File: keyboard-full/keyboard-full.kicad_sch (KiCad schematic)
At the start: 372 parts, among them SW1 SW_Push, SW10 SW_Push, SW11 SW_Push, SW12 SW_Push, SW13 SW_Push, SW14 SW_Push, SW15 SW_Push, SW16 SW_Push, SW17 SW_Push, SW18 SW_Push, SW19 SW_Push, SW2 SW_Push, SW20 SW_Push, SW21 SW_Push, SW22 SW_Push, SW23 SW_Push, SW24 SW_Push, SW25 SW_Push, SW26 SW_Push, SW27 SW_Push, SW28 SW_Push, SW29 SW_Push, SW3 SW_Push, SW30 SW_Push, SW31 SW_Push, SW32 SW_Push, SW33 SW_Push, SW34 SW_Push, SW35 SW_Push, SW36 SW_Push, SW37 SW_Push, SW38 SW_Push, SW39 SW_Push, SW4 SW_Push, SW40 SW_Push, SW41 SW_Push, SW42 SW_Push, SW43 SW_Push, SW44 SW_Push, SW45 SW_Push, SW46 SW_Push, SW47 SW_Push, SW48 SW_Push, SW49 SW_Push, SW5 SW_Push, SW50 SW_Push, SW51 SW_Push, SW52 SW_Push, SW53 SW_Push, SW54 SW_Push, SW55 SW_Push, SW56 SW_Push, SW57 SW_Push, SW58 SW_Push, SW59 SW_Push, SW6 SW_Push, SW60 SW_Push, SW61 SW_Push, SW62 SW_Push, SW63 SW_Push, SW64 SW_Push, SW65 SW_Push, SW66 SW_Push, SW67 SW_Push, SW68 SW_Push, SW69 SW_Push, SW7 SW_Push, SW70 SW_Push, SW71 SW_Push, SW72 SW_Push, SW73 SW_Push, SW74 SW_Push, SW75 SW_Push, SW76 SW_Push, SW77 SW_Push, SW78 SW_Push, SW79 SW_Push, SW8 SW_Push, SW80 SW_Push, SW81 SW_Push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

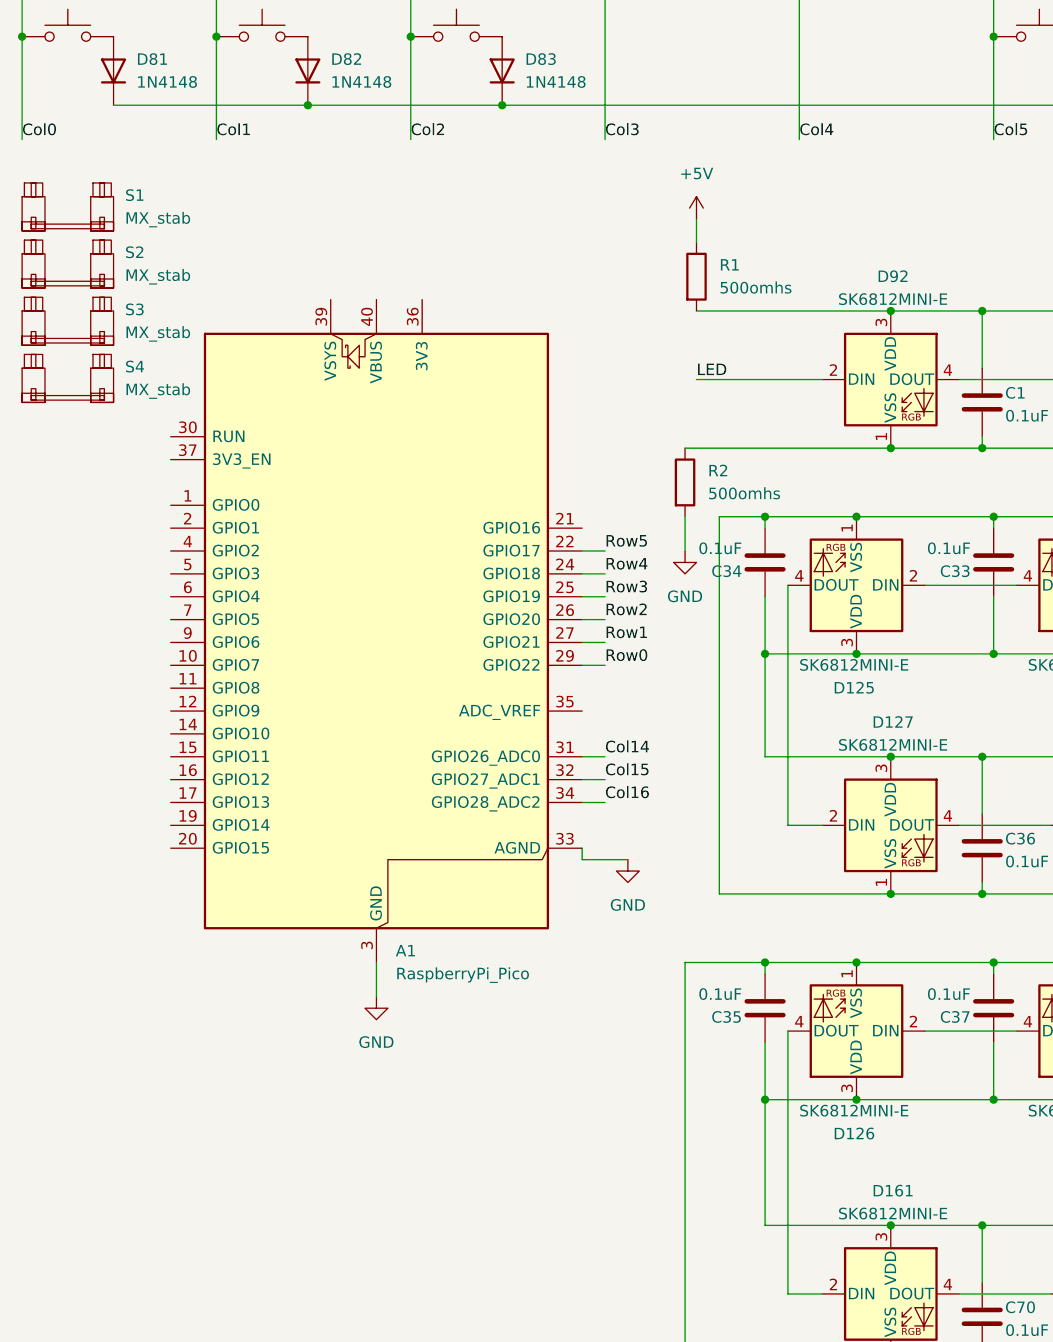
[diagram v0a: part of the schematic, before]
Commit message: Fixes to schema
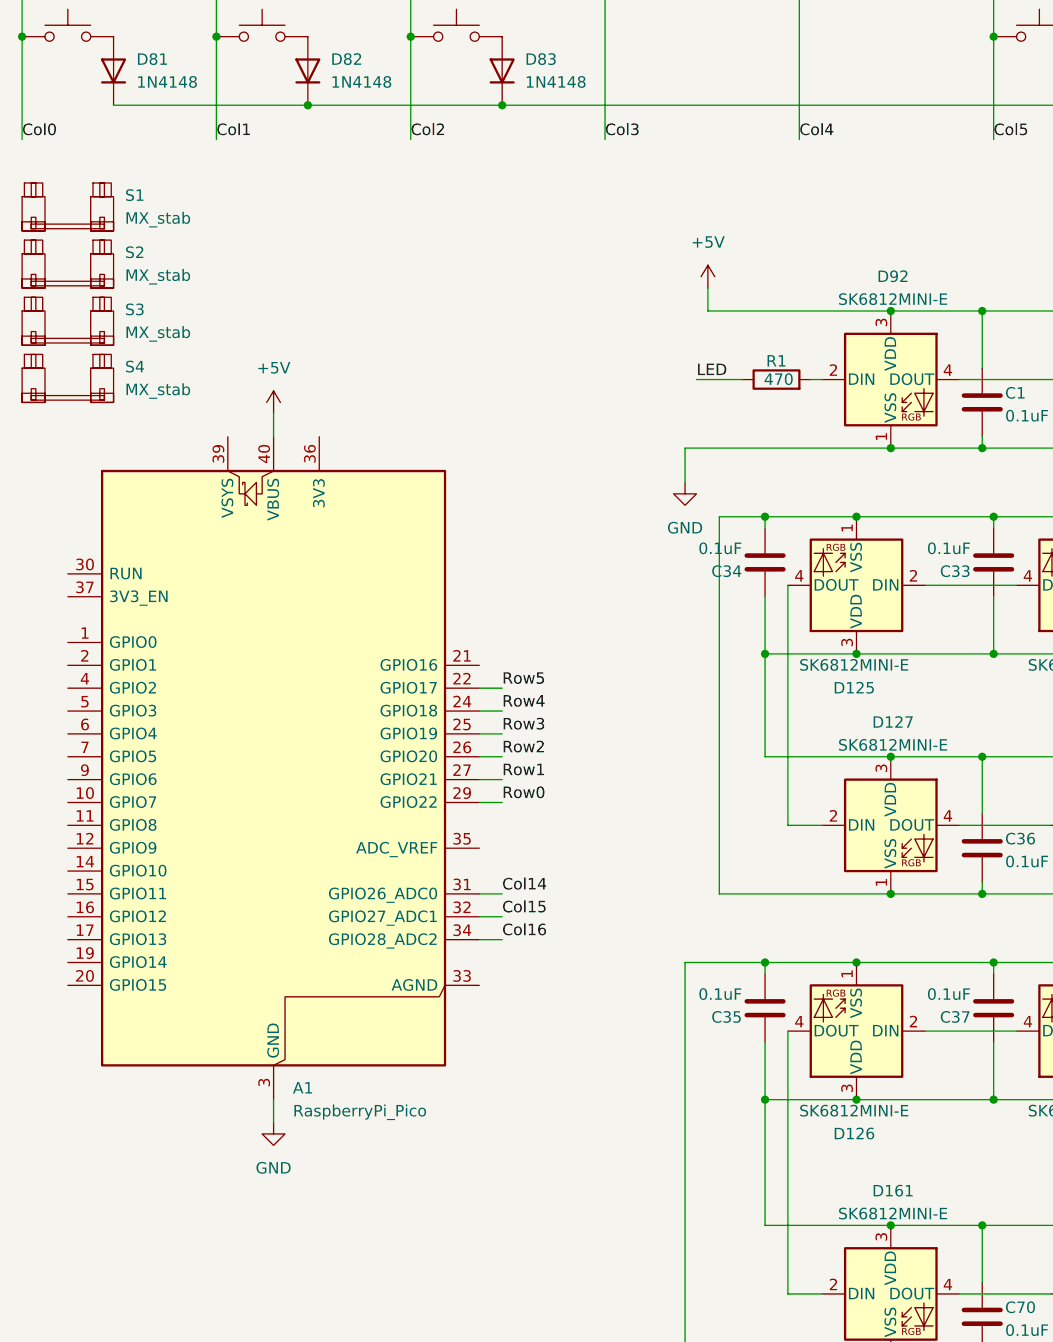
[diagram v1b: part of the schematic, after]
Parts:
- removed R2: 500omhs, symbol Device:R
- R1: value 500omhs -> 470
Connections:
- net +5V: now also A1.40 (VBUS), C1.1, C10.1, C100.1, C101.1, C102.1, C11.1, C12.1, C13.1, C14.1, C15.1, C16.1, C17.1, C18.1, C19.1, C20.1, C21.1, C22.1, C23.1, C24.1, C25.1, C26.1, C27.1, C28.1, C29.1, C3.1, C30.1, C31.1, C32.1, C33.1, C34.1, C35.1, C36.1, C37.1, C38.1, C39.1, C4.1, C40.1, C41.1, C42.1, C43.1, C44.1, C45.1, C46.1, C47.1, C48.1, C49.1, C5.1, C50.1, C51.1, C52.1, C53.1, C54.1, C55.1, C56.1, C57.1, C58.1, C59.1, C6.1, C60.1, C62.1, C63.1, C64.1, C66.1, C68.1, C69.1, C7.1, C70.1, C71.1, C72.1, C73.1, C74.1, C75.1, C76.1, C78.1, C8.1, C80.1, C81.1, C82.1, C84.1, C86.1, C88.1, C89.1, C9.1, C90.1, C91.1, C92.1, C93.1, C94.1, C96.1, C97.1, C98.1, C99.1, D100.3 (VDD), D101.3 (VDD), D102.3 (VDD), D103.3 (VDD), D104.3 (VDD), D105.3 (VDD), D106.3 (VDD), D107.3 (VDD), D108.3 (VDD), D109.3 (VDD), D110.3 (VDD), D111.3 (VDD), D112.3 (VDD), D113.3 (VDD), D114.3 (VDD), D115.3 (VDD), D116.3 (VDD), D117.3 (VDD), D118.3 (VDD), D119.3 (VDD), D120.3 (VDD), D121.3 (VDD), D122.3 (VDD), D123.3 (VDD), D124.3 (VDD), D125.3 (VDD), D126.3 (VDD), D127.3 (VDD), D128.3 (VDD), D129.3 (VDD), D130.3 (VDD), D131.3 (VDD), D132.3 (VDD), D133.3 (VDD), D134.3 (VDD), D135.3 (VDD), D136.3 (VDD), D137.3 (VDD), D138.3 (VDD), D139.3 (VDD), D140.3 (VDD), D141.3 (VDD), D142.3 (VDD), D143.3 (VDD), D144.3 (VDD), D145.3 (VDD), D146.3 (VDD), D147.3 (VDD), D148.3 (VDD), D149.3 (VDD), D151.3 (VDD), D152.3 (VDD), D153.3 (VDD), D155.3 (VDD), D157.3 (VDD), D159.3 (VDD), D160.3 (VDD), D161.3 (VDD), D162.3 (VDD), D163.3 (VDD), D164.3 (VDD), D165.3 (VDD), D167.3 (VDD), D169.3 (VDD), D170.3 (VDD), D171.3 (VDD), D173.3 (VDD), D175.3 (VDD), D177.3 (VDD), D178.3 (VDD), D179.3 (VDD), D180.3 (VDD), D181.3 (VDD), D182.3 (VDD), D183.3 (VDD), D185.3 (VDD), D186.3 (VDD), D187.3 (VDD), D188.3 (VDD), D189.3 (VDD), D190.3 (VDD), D191.3 (VDD), D192.3 (VDD), D193.3 (VDD), D92.3 (VDD), D94.3 (VDD), D95.3 (VDD), D96.3 (VDD), D97.3 (VDD), D98.3 (VDD), D99.3 (VDD); no longer R1.1
- net GND: now also C1.2, C10.2, C100.2, C101.2, C102.2, C11.2, C12.2, C13.2, C14.2, C15.2, C16.2, C17.2, C18.2, C19.2, C20.2, C21.2, C22.2, C23.2, C24.2, C25.2, C26.2, C27.2, C28.2, C29.2, C3.2, C30.2, C31.2, C32.2, C33.2, C34.2, C35.2, C36.2, C37.2, C38.2, C39.2, C4.2, C40.2, C41.2, C42.2, C43.2, C44.2, C45.2, C46.2, C47.2, C48.2, C49.2, C5.2, C50.2, C51.2, C52.2, C53.2, C54.2, C55.2, C56.2, C57.2, C58.2, C59.2, C6.2, C60.2, C62.2, C63.2, C64.2, C66.2, C68.2, C69.2, C7.2, C70.2, C71.2, C72.2, C73.2, C74.2, C75.2, C76.2, C78.2, C8.2, C80.2, C81.2, C82.2, C84.2, C86.2, C88.2, C89.2, C9.2, C90.2, C91.2, C92.2, C93.2, C94.2, C96.2, C97.2, C98.2, C99.2, D100.1 (VSS), D101.1 (VSS), D102.1 (VSS), D103.1 (VSS), D104.1 (VSS), D105.1 (VSS), D106.1 (VSS), D107.1 (VSS), D108.1 (VSS), D109.1 (VSS), D110.1 (VSS), D111.1 (VSS), D112.1 (VSS), D113.1 (VSS), D114.1 (VSS), D115.1 (VSS), D116.1 (VSS), D117.1 (VSS), D118.1 (VSS), D119.1 (VSS), D120.1 (VSS), D121.1 (VSS), D122.1 (VSS), D123.1 (VSS), D124.1 (VSS), D125.1 (VSS), D126.1 (VSS), D127.1 (VSS), D128.1 (VSS), D129.1 (VSS), D130.1 (VSS), D131.1 (VSS), D132.1 (VSS), D133.1 (VSS), D134.1 (VSS), D135.1 (VSS), D136.1 (VSS), D137.1 (VSS), D138.1 (VSS), D139.1 (VSS), D140.1 (VSS), D141.1 (VSS), D142.1 (VSS), D143.1 (VSS), D144.1 (VSS), D145.1 (VSS), D146.1 (VSS), D147.1 (VSS), D148.1 (VSS), D149.1 (VSS), D151.1 (VSS), D152.1 (VSS), D153.1 (VSS), D155.1 (VSS), D157.1 (VSS), D159.1 (VSS), D160.1 (VSS), D161.1 (VSS), D162.1 (VSS), D163.1 (VSS), D164.1 (VSS), D165.1 (VSS), D167.1 (VSS), D169.1 (VSS), D170.1 (VSS), D171.1 (VSS), D173.1 (VSS), D175.1 (VSS), D177.1 (VSS), D178.1 (VSS), D179.1 (VSS), D180.1 (VSS), D181.1 (VSS), D182.1 (VSS), D183.1 (VSS), D185.1 (VSS), D186.1 (VSS), D187.1 (VSS), D188.1 (VSS), D189.1 (VSS), D190.1 (VSS), D191.1 (VSS), D192.1 (VSS), D193.1 (VSS), D92.1 (VSS), D94.1 (VSS), D95.1 (VSS), D96.1 (VSS), D97.1 (VSS), D98.1 (VSS), D99.1 (VSS); no longer A1.33 (AGND)
- net LED: now also R1.1; no longer D92.2 (DIN)
- new net: D92.2 (DIN), R1.2
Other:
- moved on the sheet: A1

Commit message: progress on keyboard
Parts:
- removed C100, C101, C102, C92, C93, C94, C96, C97, C98, C99: 0.1uF, symbol Device:C
- removed D109, D110, D111, D112, D113, D114, D115, D116, D117, D118, D119, D120, D121, D122, D123, D124, D125, D126, D127, D128, D129, D130, D131, D132, D133, D134, D135, D136, D137, D138, D139, D140, D141, D142, D143, D144, D145, D146, D147, D148, D149, D151, D152, D153, D155, D157, D159, D160, D161, D162, D163, D164, D165, D167, D169, D170, D171, D173, D175, D177, D178, D179, D180, D181, D182, D183, D185, D186, D187, D188, D189, D190, D191, D192, D193: SK6812MINI-E, LED_SMD:LED_SK6812MINI-E_3.2x2.8mm_P1.5mm_ReverseMount, symbol LED:SK6812MINI-E
- removed SW1, SW10, SW11, SW12, SW13, SW14, SW15, SW16, SW17, SW18, SW19, SW2, SW20, SW21, SW22, SW23, SW24, SW25, SW26, SW27, SW28, SW29, SW3, SW30, SW31, SW32, SW33, SW34, SW35, SW36, SW37, SW38, SW39, SW4, SW40, SW41, SW42, SW43, SW44, SW45, SW46, SW47, SW48, SW49, SW5, SW50, SW51, SW52, SW53, SW54, SW55, SW56, SW57, SW58, SW59, SW6, SW60, SW61, SW62, SW63, SW64, SW65, SW66, SW67, SW68, SW69, SW7, SW70, SW71, SW72, SW73, SW74, SW75, SW76, SW77, SW78, SW79, SW8, SW80, SW81, SW82, SW83, SW85, SW86, SW87, SW88, SW89, SW9, SW90, SW91: SW_Push, PCM_marbastlib-mx:SW_MX_1u, symbol Switch:SW_Push
- removed SW84: SW_Push, PCM_marbastlib-mx:STAB_MX_P_6u, symbol Switch:SW_Push
- added C17, C61, C65, C67, C77, C79, C83, C85, C87: 0.1uF, Capacitor_SMD:C_1206_3216Metric_Pad1.33x1.80mm_HandSolder, symbol Device:C
- added H1, H2, H3, H4: MountingHole, MountingHole:MountingHole_2.1mm, symbol Mechanical:MountingHole
- added LED17, LED18, LED19, LED20, LED21, LED22, LED23, LED24, LED25, LED26, LED27, LED28, LED29, LED30, LED31, LED32, LED33, LED34, LED35, LED36, LED37, LED38, LED39, LED40, LED41, LED42, LED43, LED44, LED45, LED46, LED47, LED48, LED49, LED50, LED51, LED52, LED53, LED54, LED55, LED56, LED57, LED58, LED59, LED60, LED61, LED62, LED63, LED64, LED65, LED66, LED67, LED68, LED69, LED70, LED71, LED72, LED73, LED74, LED75, LED76, LED77, LED78, LED79, LED80, LED81, LED82, LED83, LED84, LED85, LED86, LED87, LED88, LED89, LED90, LED91: SK6812MINI-E, LED_SMD:LED_SK6812MINI-E_3.2x2.8mm_P1.5mm_ReverseMount, symbol LED:SK6812MINI-E
- added MX1, MX10, MX11, MX12, MX13, MX14, MX15, MX16, MX17, MX18, MX19, MX2, MX20, MX21, MX22, MX23, MX24, MX25, MX26, MX27, MX28, MX29, MX3, MX30, MX31, MX32, MX33, MX35, MX36, MX37, MX38, MX39, MX4, MX40, MX41, MX42, MX43, MX44, MX45, MX46, MX48, MX49, MX5, MX50, MX52, MX53, MX54, MX55, MX56, MX57, MX58, MX59, MX6, MX60, MX61, MX62, MX63, MX64, MX65, MX66, MX67, MX68, MX69, MX7, MX70, MX71, MX72, MX73, MX74, MX75, MX76, MX77, MX78, MX79, MX8, MX80, MX89, MX9, MX90, MX91: MX_SW_HS, PCM_marbastlib-mx:SW_MX_HS_CPG151101S11_1u, symbol PCM_marbastlib-mx:MX_SW_HS_CPG151101S11
- added MX34: MX_SW_HS, PCM_marbastlib-mx:SW_MX_HS_CPG151101S11_1.5u, symbol PCM_marbastlib-mx:MX_SW_HS_CPG151101S11
- added MX47: MX_SW_HS, PCM_marbastlib-mx:SW_MX_HS_KS-2P02B01-01_1.5u, symbol PCM_marbastlib-mx:MX_SW_HS_CPG151101S11
- added MX51: MX_SW_HS, PCM_marbastlib-mx:SW_MX_HS_KS-2P02B01-01_1.75u, symbol PCM_marbastlib-mx:MX_SW_HS_CPG151101S11
- added MX81, MX82, MX83, MX85, MX86, MX87, MX88: MX_SW_HS, PCM_marbastlib-mx:SW_MX_HS_KS-2P02B01-01_1.25u, symbol PCM_marbastlib-mx:MX_SW_HS_CPG151101S11
- added MX84: MX_SW_HS, PCM_marbastlib-mx:SW_MX_HS_CPG151101S11_1.25u, symbol PCM_marbastlib-mx:MX_SW_HS_CPG151101S11
- C1, C18, C19, C20, C21, C22, C23, C24, C25, C26, C27, C28, C29, C30, C31, C32, C33, C34, C35, C36, C37, C38, C39, C40, C41, C42, C43, C44, C45, C46, C47, C48, C49, C50, C51, C52, C53, C54, C55, C56, C57, C58, C59, C60, C62, C63, C64, C66, C68, C69, C70, C71, C72, C73, C74, C75, C76, C78, C80, C81, C82, C84, C86, C88, C89, C90, C91: footprint (none) -> Capacitor_SMD:C_1206_3216Metric_Pad1.33x1.80mm_HandSolder
- C10: renamed from C11; footprint (none) -> Capacitor_SMD:C_1206_3216Metric_Pad1.33x1.80mm_HandSolder
- C11: renamed from C12; footprint (none) -> Capacitor_SMD:C_1206_3216Metric_Pad1.33x1.80mm_HandSolder
- C12: renamed from C13; footprint (none) -> Capacitor_SMD:C_1206_3216Metric_Pad1.33x1.80mm_HandSolder
- C13: renamed from C14; footprint (none) -> Capacitor_SMD:C_1206_3216Metric_Pad1.33x1.80mm_HandSolder
- C14: renamed from C15; footprint (none) -> Capacitor_SMD:C_1206_3216Metric_Pad1.33x1.80mm_HandSolder
- C15: renamed from C16; footprint (none) -> Capacitor_SMD:C_1206_3216Metric_Pad1.33x1.80mm_HandSolder
- C16: renamed from C17; footprint (none) -> Capacitor_SMD:C_1206_3216Metric_Pad1.33x1.80mm_HandSolder
- C2: renamed from C3; footprint (none) -> Capacitor_SMD:C_1206_3216Metric_Pad1.33x1.80mm_HandSolder
- C3: renamed from C4; footprint (none) -> Capacitor_SMD:C_1206_3216Metric_Pad1.33x1.80mm_HandSolder
- C4: renamed from C5; footprint (none) -> Capacitor_SMD:C_1206_3216Metric_Pad1.33x1.80mm_HandSolder
- C5: renamed from C6; footprint (none) -> Capacitor_SMD:C_1206_3216Metric_Pad1.33x1.80mm_HandSolder
- C6: renamed from C7; footprint (none) -> Capacitor_SMD:C_1206_3216Metric_Pad1.33x1.80mm_HandSolder
- C7: renamed from C8; footprint (none) -> Capacitor_SMD:C_1206_3216Metric_Pad1.33x1.80mm_HandSolder
- C8: renamed from C9; footprint (none) -> Capacitor_SMD:C_1206_3216Metric_Pad1.33x1.80mm_HandSolder
- C9: renamed from C10; footprint (none) -> Capacitor_SMD:C_1206_3216Metric_Pad1.33x1.80mm_HandSolder
- R1: footprint (none) -> Resistor_THT:R_Axial_DIN0207_L6.3mm_D2.5mm_P7.62mm_Horizontal
- S2, S3: footprint PCM_marbastlib-mx:STAB_MX_P_6.25u -> PCM_marbastlib-mx:STAB_MX_2u
- S4: footprint PCM_marbastlib-mx:STAB_MX_P_6.25u -> PCM_marbastlib-mx:STAB_MX_2.25u
- renumbered D92 to LED1, D102 to LED10, D103 to LED11, D104 to LED12, D105 to LED13, D106 to LED14, D107 to LED15, D108 to LED16, D94 to LED2, D95 to LED3, D96 to LED4, D97 to LED5, D98 to LED6, D99 to LED7, D100 to LED8, D101 to LED9
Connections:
- net +5V: now also C17.1, C61.1, C65.1, C67.1, C77.1, C79.1, C83.1, C85.1, C87.1, LED17.3 (VDD), LED18.3 (VDD), LED19.3 (VDD), LED20.3 (VDD), LED21.3 (VDD), LED22.3 (VDD), LED23.3 (VDD), LED24.3 (VDD), LED25.3 (VDD), LED26.3 (VDD), LED27.3 (VDD), LED28.3 (VDD), LED29.3 (VDD), LED30.3 (VDD), LED31.3 (VDD), LED32.3 (VDD), LED33.3 (VDD), LED34.3 (VDD), LED35.3 (VDD), LED36.3 (VDD), LED37.3 (VDD), LED38.3 (VDD), LED39.3 (VDD), LED40.3 (VDD), LED41.3 (VDD), LED42.3 (VDD), LED43.3 (VDD), LED44.3 (VDD), LED45.3 (VDD), LED46.3 (VDD), LED47.3 (VDD), LED48.3 (VDD), LED49.3 (VDD), LED50.3 (VDD), LED51.3 (VDD), LED52.3 (VDD), LED53.3 (VDD), LED54.3 (VDD), LED55.3 (VDD), LED56.3 (VDD), LED57.3 (VDD), LED58.3 (VDD), LED59.3 (VDD), LED60.3 (VDD), LED61.3 (VDD), LED62.3 (VDD), LED63.3 (VDD), LED64.3 (VDD), LED65.3 (VDD), LED66.3 (VDD), LED67.3 (VDD), LED68.3 (VDD), LED69.3 (VDD), LED70.3 (VDD), LED71.3 (VDD), LED72.3 (VDD), LED73.3 (VDD), LED74.3 (VDD), LED75.3 (VDD), LED76.3 (VDD), LED77.3 (VDD), LED78.3 (VDD), LED79.3 (VDD), LED80.3 (VDD), LED81.3 (VDD), LED82.3 (VDD), LED83.3 (VDD), LED84.3 (VDD), LED85.3 (VDD), LED86.3 (VDD), LED87.3 (VDD), LED88.3 (VDD), LED89.3 (VDD), LED90.3 (VDD), LED91.3 (VDD)
- net Col0: now also MX1.1, MX17.1, MX34.1, MX51.1, MX64.1, MX81.1
- net Col1: now also MX18.1, MX35.1, MX52.1, MX65.1, MX82.1
- net Col10: now also MX10.1, MX27.1, MX44.1, MX61.1, MX74.1, MX86.1
- net Col11: now also MX11.1, MX28.1, MX45.1, MX62.1, MX75.1, MX87.1
- net Col12: now also MX12.1, MX29.1, MX46.1, MX76.1
- net Col13: now also MX13.1, MX30.1, MX47.1, MX63.1, MX77.1, MX88.1
- net Col14: now also MX14.1, MX31.1, MX48.1, MX78.1, MX89.1
- net Col15: now also MX15.1, MX32.1, MX49.1, MX79.1, MX90.1
- net Col16: now also MX16.1, MX33.1, MX50.1, MX80.1, MX91.1
- net Col2: now also MX19.1, MX2.1, MX36.1, MX53.1, MX66.1, MX83.1
- net Col3: now also MX20.1, MX3.1, MX37.1, MX54.1, MX67.1
- net Col4: now also MX21.1, MX38.1, MX4.1, MX55.1, MX68.1
- net Col5: now also MX22.1, MX39.1, MX5.1, MX56.1, MX69.1, MX84.1
- net Col6: now also MX23.1, MX40.1, MX57.1, MX6.1, MX70.1
- net Col7: now also MX24.1, MX41.1, MX58.1, MX7.1, MX71.1
- net Col8: now also MX25.1, MX42.1, MX59.1, MX72.1, MX8.1
- net Col9: now also MX26.1, MX43.1, MX60.1, MX73.1, MX85.1, MX9.1
- net GND: now also C17.2, C61.2, C65.2, C67.2, C77.2, C79.2, C83.2, C85.2, C87.2, LED17.1 (VSS), LED18.1 (VSS), LED19.1 (VSS), LED20.1 (VSS), LED21.1 (VSS), LED22.1 (VSS), LED23.1 (VSS), LED24.1 (VSS), LED25.1 (VSS), LED26.1 (VSS), LED27.1 (VSS), LED28.1 (VSS), LED29.1 (VSS), LED30.1 (VSS), LED31.1 (VSS), LED32.1 (VSS), LED33.1 (VSS), LED34.1 (VSS), LED35.1 (VSS), LED36.1 (VSS), LED37.1 (VSS), LED38.1 (VSS), LED39.1 (VSS), LED40.1 (VSS), LED41.1 (VSS), LED42.1 (VSS), LED43.1 (VSS), LED44.1 (VSS), LED45.1 (VSS), LED46.1 (VSS), LED47.1 (VSS), LED48.1 (VSS), LED49.1 (VSS), LED50.1 (VSS), LED51.1 (VSS), LED52.1 (VSS), LED53.1 (VSS), LED54.1 (VSS), LED55.1 (VSS), LED56.1 (VSS), LED57.1 (VSS), LED58.1 (VSS), LED59.1 (VSS), LED60.1 (VSS), LED61.1 (VSS), LED62.1 (VSS), LED63.1 (VSS), LED64.1 (VSS), LED65.1 (VSS), LED66.1 (VSS), LED67.1 (VSS), LED68.1 (VSS), LED69.1 (VSS), LED70.1 (VSS), LED71.1 (VSS), LED72.1 (VSS), LED73.1 (VSS), LED74.1 (VSS), LED75.1 (VSS), LED76.1 (VSS), LED77.1 (VSS), LED78.1 (VSS), LED79.1 (VSS), LED80.1 (VSS), LED81.1 (VSS), LED82.1 (VSS), LED83.1 (VSS), LED84.1 (VSS), LED85.1 (VSS), LED86.1 (VSS), LED87.1 (VSS), LED88.1 (VSS), LED89.1 (VSS), LED90.1 (VSS), LED91.1 (VSS)
- net at D30.2 (A): now also MX30.2
- net at D86.2 (A): now also MX86.2
- net at D36.2 (A): now also MX36.2
- net at D68.2 (A): now also MX68.2
- net at D78.2 (A): now also MX78.2
- net at D21.2 (A): now also MX21.2
- net at D72.2 (A): now also MX72.2
- net at D35.2 (A): now also MX35.2
- net at D54.2 (A): now also MX54.2
- net at D81.2 (A): now also MX81.2
- net at D62.2 (A): now also MX62.2
- net at D70.2 (A): now also MX70.2
- net at D29.2 (A): now also MX29.2
- net at D57.2 (A): now also MX57.2
- net at D76.2 (A): now also MX76.2
- net at D56.2 (A): now also MX56.2
- net at D26.2 (A): now also MX26.2
- net at D88.2 (A): now also MX88.2
- net at D66.2 (A): now also MX66.2
- net at D6.2 (A): now also MX6.2
- net at D49.2 (A): now also MX49.2
- net at D1.2 (A): now also MX1.2
- net at D33.2 (A): now also MX33.2
- net at D37.2 (A): now also MX37.2
- net at D48.2 (A): now also MX48.2
- net at D75.2 (A): now also MX75.2
- net at D90.2 (A): now also MX90.2
- net at D79.2 (A): now also MX79.2
- net at D74.2 (A): now also MX74.2
- net at D22.2 (A): now also MX22.2
- net at D28.2 (A): now also MX28.2
- net at D15.2 (A): now also MX15.2
- net at D2.2 (A): now also MX2.2
- net at D85.2 (A): now also MX85.2
- net at D23.2 (A): now also MX23.2
- net at D7.2 (A): now also MX7.2
- net at D55.2 (A): now also MX55.2
- net at D9.2 (A): now also MX9.2
- net at D44.2 (A): now also MX44.2
- net at D41.2 (A): now also MX41.2
- net at D67.2 (A): now also MX67.2
- net at D65.2 (A): now also MX65.2
- net at D77.2 (A): now also MX77.2
- net at D17.2 (A): now also MX17.2
- net at D31.2 (A): now also MX31.2
- net at D8.2 (A): now also MX8.2
- net at D91.2 (A): now also MX91.2
- net at D34.2 (A): now also MX34.2
- net at D27.2 (A): now also MX27.2
- net at D4.2 (A): now also MX4.2
- net at D32.2 (A): now also MX32.2
- net at D24.2 (A): now also MX24.2
- net at D38.2 (A): now also MX38.2
- net at D5.2 (A): now also MX5.2
- net at D89.2 (A): now also MX89.2
- net at D50.2 (A): now also MX50.2
- net at D42.2 (A): now also MX42.2
- net at LED16.4 (DOUT): now also LED17.2 (DIN)
- net at D59.2 (A): now also MX59.2
- net at D10.2 (A): now also MX10.2
- net at D69.2 (A): now also MX69.2
- net at D73.2 (A): now also MX73.2
- net at D46.2 (A): now also MX46.2
- net at D13.2 (A): now also MX13.2
- net at D53.2 (A): now also MX53.2
- net at D12.2 (A): now also MX12.2
- net at D52.2 (A): now also MX52.2
- net at D84.2 (A): now also MX84.2
- net at D45.2 (A): now also MX45.2
- net at D58.2 (A): now also MX58.2
- net at D83.2 (A): now also MX83.2
- net at D3.2 (A): now also MX3.2
- net at D39.2 (A): now also MX39.2
- net at D47.2 (A): now also MX47.2
- net at D11.2 (A): now also MX11.2
- net at D71.2 (A): now also MX71.2
- net at D61.2 (A): now also MX61.2
- net at D63.2 (A): now also MX63.2
- net at D82.2 (A): now also MX82.2
- net at D51.2 (A): now also MX51.2
- net at D14.2 (A): now also MX14.2
- net at D25.2 (A): now also MX25.2
- net at D18.2 (A): now also MX18.2
- net at D19.2 (A): now also MX19.2
- net at D60.2 (A): now also MX60.2
- net at D40.2 (A): now also MX40.2
- net at D87.2 (A): now also MX87.2
- net at D16.2 (A): now also MX16.2
- net at D64.2 (A): now also MX64.2
- net at D80.2 (A): now also MX80.2
- net at D20.2 (A): now also MX20.2
- net at D43.2 (A): now also MX43.2
- new net: LED42.4 (DOUT), LED43.2 (DIN)
- new net: LED43.4 (DOUT), LED44.2 (DIN)
- new net: LED38.4 (DOUT), LED39.2 (DIN)
- new net: LED39.4 (DOUT), LED40.2 (DIN)
- new net: LED60.4 (DOUT), LED61.2 (DIN)
- new net: LED61.4 (DOUT), LED62.2 (DIN)
- new net: LED64.4 (DOUT), LED65.2 (DIN)
- new net: LED65.4 (DOUT), LED66.2 (DIN)
- new net: LED62.4 (DOUT), LED63.2 (DIN)
- new net: LED63.4 (DOUT), LED64.2 (DIN)
- new net: LED24.4 (DOUT), LED25.2 (DIN)
- new net: LED25.4 (DOUT), LED26.2 (DIN)
- new net: LED47.4 (DOUT), LED48.2 (DIN)
- new net: LED48.4 (DOUT), LED49.2 (DIN)
- new net: LED35.4 (DOUT), LED36.2 (DIN)
- new net: LED36.4 (DOUT), LED37.2 (DIN)
- new net: LED22.4 (DOUT), LED23.2 (DIN)
- new net: LED23.4 (DOUT), LED24.2 (DIN)
- new net: LED76.4 (DOUT), LED77.2 (DIN)
- new net: LED77.4 (DOUT), LED78.2 (DIN)
- new net: LED89.4 (DOUT), LED90.2 (DIN)
- new net: LED90.4 (DOUT), LED91.2 (DIN)
- new net: LED66.4 (DOUT), LED67.2 (DIN)
- new net: LED67.4 (DOUT), LED68.2 (DIN)
- new net: LED85.4 (DOUT), LED86.2 (DIN)
- new net: LED86.4 (DOUT), LED87.2 (DIN)
- new net: LED57.4 (DOUT), LED58.2 (DIN)
- new net: LED58.4 (DOUT), LED59.2 (DIN)
- new net: LED20.4 (DOUT), LED21.2 (DIN)
- new net: LED21.4 (DOUT), LED22.2 (DIN)
- new net: LED40.4 (DOUT), LED41.2 (DIN)
- new net: LED44.4 (DOUT), LED45.2 (DIN)
- new net: LED45.4 (DOUT), LED46.2 (DIN)
- new net: LED50.4 (DOUT), LED51.2 (DIN)
- new net: LED51.4 (DOUT), LED52.2 (DIN)
- new net: LED26.4 (DOUT), LED27.2 (DIN)
- new net: LED27.4 (DOUT), LED28.2 (DIN)
- new net: LED46.4 (DOUT), LED47.2 (DIN)
- new net: LED87.4 (DOUT), LED88.2 (DIN)
- new net: LED17.4 (DOUT), LED18.2 (DIN)
- new net: LED41.4 (DOUT), LED42.2 (DIN)
- new net: LED82.4 (DOUT), LED83.2 (DIN)
- new net: LED83.4 (DOUT), LED84.2 (DIN)
- new net: LED28.4 (DOUT), LED29.2 (DIN)
- new net: LED37.4 (DOUT), LED38.2 (DIN)
- new net: LED78.4 (DOUT), LED79.2 (DIN)
- new net: LED59.4 (DOUT), LED60.2 (DIN)
- new net: LED68.4 (DOUT), LED69.2 (DIN)
- new net: LED54.4 (DOUT), LED55.2 (DIN)
- new net: LED55.4 (DOUT), LED56.2 (DIN)
- new net: LED19.4 (DOUT), LED20.2 (DIN)
- new net: LED79.4 (DOUT), LED80.2 (DIN)
- new net: LED80.4 (DOUT), LED81.2 (DIN)
- new net: LED81.4 (DOUT), LED82.2 (DIN)
- new net: LED71.4 (DOUT), LED72.2 (DIN)
- new net: LED72.4 (DOUT), LED73.2 (DIN)
- new net: LED33.4 (DOUT), LED34.2 (DIN)
- new net: LED34.4 (DOUT), LED35.2 (DIN)
- new net: LED70.4 (DOUT), LED71.2 (DIN)
- new net: LED49.4 (DOUT), LED50.2 (DIN)
- new net: LED56.4 (DOUT), LED57.2 (DIN)
- new net: LED53.4 (DOUT), LED54.2 (DIN)
- new net: LED84.4 (DOUT), LED85.2 (DIN)
- new net: LED18.4 (DOUT), LED19.2 (DIN)
- new net: LED75.4 (DOUT), LED76.2 (DIN)
- new net: LED73.4 (DOUT), LED74.2 (DIN)
- new net: LED74.4 (DOUT), LED75.2 (DIN)
- new net: LED30.4 (DOUT), LED31.2 (DIN)
- new net: LED31.4 (DOUT), LED32.2 (DIN)
- new net: LED69.4 (DOUT), LED70.2 (DIN)
- new net: LED32.4 (DOUT), LED33.2 (DIN)
- new net: LED52.4 (DOUT), LED53.2 (DIN)
- new net: LED29.4 (DOUT), LED30.2 (DIN)
- new net: LED88.4 (DOUT), LED89.2 (DIN)
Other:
- moved on the sheet: A1, C1, C10, C11, C12, C13, C14, C15, C16, C2, C3, C4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

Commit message: Started wiring, and fixed pcb's rgbs data line going across the whole board
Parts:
- added C100, C101, C102, C92, C93, C94, C95, C96, C97, C98, C99: 0.1uF, Capacitor_SMD:C_1206_3216Metric_Pad1.33x1.80mm_HandSolder, symbol Device:C
- added LED100, LED101, LED102, LED92, LED93, LED94, LED95, LED96, LED97, LED98, LED99: SK6812MINI-E, LED_SMD:LED_SK6812MINI-E_3.2x2.8mm_P1.5mm_ReverseMount, symbol LED:SK6812MINI-E
- S1: footprint PCM_marbastlib-mx:STAB_MX_P_6.25u -> PCM_marbastlib-mx:STAB_MX_6.25u
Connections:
- net +5V: now also C100.1, C101.1, C102.1, C92.1, C93.1, C94.1, C95.1, C96.1, C97.1, C98.1, C99.1, LED100.3 (VDD), LED101.3 (VDD), LED102.3 (VDD), LED92.3 (VDD), LED93.3 (VDD), LED94.3 (VDD), LED95.3 (VDD), LED96.3 (VDD), LED97.3 (VDD), LED98.3 (VDD), LED99.3 (VDD)
- net GND: now also C100.2, C101.2, C102.2, C92.2, C93.2, C94.2, C95.2, C96.2, C97.2, C98.2, C99.2, LED100.1 (VSS), LED101.1 (VSS), LED102.1 (VSS), LED92.1 (VSS), LED93.1 (VSS), LED94.1 (VSS), LED95.1 (VSS), LED96.1 (VSS), LED97.1 (VSS), LED98.1 (VSS), LED99.1 (VSS)
- net at LED43.2 (DIN): now also LED41.4 (DOUT); no longer LED42.4 (DOUT)
- net at LED43.4 (DOUT): now also LED45.2 (DIN); no longer LED44.2 (DIN)
- net at LED38.4 (DOUT): now also LED36.2 (DIN); no longer LED39.2 (DIN)
- net at LED39.4 (DOUT): now also LED41.2 (DIN); no longer LED40.2 (DIN)
- net at LED60.4 (DOUT): now also LED58.2 (DIN); no longer LED61.2 (DIN)
- net at LED62.2 (DIN): now also LED64.4 (DOUT); no longer LED61.4 (DOUT)
- net at LED1.4 (DOUT): now also LED17.2 (DIN); no longer LED2.2 (DIN)
- net at LED65.2 (DIN): now also LED63.4 (DOUT); no longer LED64.4 (DOUT)
- net at LED66.2 (DIN): now also LED68.4 (DOUT); no longer LED65.4 (DOUT)
- net at LED62.4 (DOUT): now also LED60.2 (DIN); no longer LED63.2 (DIN)
- net at LED64.2 (DIN): now also LED66.4 (DOUT); no longer LED63.4 (DOUT)
- net at LED48.2 (DIN): now also LED50.4 (DOUT); no longer LED47.4 (DOUT)
- net at LED48.4 (DOUT): now also LED46.2 (DIN); no longer LED49.2 (DIN)
- net at LED35.4 (DOUT): now also LED37.2 (DIN); no longer LED36.2 (DIN)
- net at LED36.4 (DOUT): now also LED69.2 (DIN); no longer LED37.2 (DIN)
- net at LED76.4 (DOUT): now also LED74.2 (DIN); no longer LED77.2 (DIN)
- net at LED77.4 (DOUT): now also LED79.2 (DIN); no longer LED78.2 (DIN)
- net at LED89.4 (DOUT): now also LED91.2 (DIN); no longer LED90.2 (DIN)
- net at LED90.4 (DOUT): now also LED88.2 (DIN); no longer LED91.2 (DIN)
- net at LED67.2 (DIN): now also LED65.4 (DOUT); no longer LED66.4 (DOUT)
- net at LED86.2 (DIN): now also LED88.4 (DOUT); no longer LED85.4 (DOUT)
- net at LED86.4 (DOUT): now also LED84.2 (DIN); no longer LED87.2 (DIN)
- net at LED57.4 (DOUT): now also LED59.2 (DIN); no longer LED58.2 (DIN)
- net at LED58.4 (DOUT): now also LED56.2 (DIN); no longer LED59.2 (DIN)
- net at LED40.4 (DOUT): now also LED38.2 (DIN); no longer LED41.2 (DIN)
- net at LED44.4 (DOUT): now also LED42.2 (DIN); no longer LED45.2 (DIN)
- net at LED45.4 (DOUT): now also LED47.2 (DIN); no longer LED46.2 (DIN)
- net at LED51.2 (DIN): now also LED49.4 (DOUT); no longer LED50.4 (DOUT)
- net at LED52.2 (DIN): now also LED54.4 (DOUT); no longer LED51.4 (DOUT)
- net at LED46.4 (DOUT): now also LED44.2 (DIN); no longer LED47.2 (DIN)
- net at LED87.4 (DOUT): now also LED89.2 (DIN); no longer LED88.2 (DIN)
- net at LED16.4 (DOUT): now also LED18.2 (DIN); no longer LED17.2 (DIN)
- net at LED17.4 (DOUT): now also LED2.2 (DIN); no longer LED18.2 (DIN)
- net at LED83.2 (DIN): now also LED81.4 (DOUT); no longer LED82.4 (DOUT)
- net at LED83.4 (DOUT): now also LED85.2 (DIN); no longer LED84.2 (DIN)
- net at LED37.4 (DOUT): now also LED39.2 (DIN); no longer LED38.2 (DIN)
- net at LED91.4 (DOUT): now also LED93.2 (DIN)
- net at LED78.4 (DOUT): now also LED76.2 (DIN); no longer LED79.2 (DIN)
- net at LED59.4 (DOUT): now also LED61.2 (DIN); no longer LED60.2 (DIN)
- net at LED55.2 (DIN): now also LED53.4 (DOUT); no longer LED54.4 (DOUT)
- net at LED55.4 (DOUT): now also LED57.2 (DIN); no longer LED56.2 (DIN)
- net at LED79.4 (DOUT): now also LED81.2 (DIN); no longer LED80.2 (DIN)
- net at LED80.4 (DOUT): now also LED78.2 (DIN); no longer LED81.2 (DIN)
- net at LED82.2 (DIN): now also LED84.4 (DOUT); no longer LED81.4 (DOUT)
- net at LED72.2 (DIN): now also LED74.4 (DOUT); no longer LED71.4 (DOUT)
- net at LED72.4 (DOUT): now also LED70.2 (DIN); no longer LED73.2 (DIN)
- net at LED70.4 (DOUT): no longer LED71.2 (DIN)
- net at LED50.2 (DIN): now also LED52.4 (DOUT); no longer LED49.4 (DOUT)
- net at LED56.4 (DOUT): now also LED54.2 (DIN); no longer LED57.2 (DIN)
- net at LED75.4 (DOUT): now also LED77.2 (DIN); no longer LED76.2 (DIN)
- net at LED73.4 (DOUT): now also LED75.2 (DIN); no longer LED74.2 (DIN)
- net at LED69.4 (DOUT): now also LED71.2 (DIN); no longer LED70.2 (DIN)
- net at LED53.2 (DIN): now also LED51.4 (DOUT); no longer LED52.4 (DOUT)
- new net: LED93.4 (DOUT), LED95.2 (DIN)
- new net: LED95.4 (DOUT), LED97.2 (DIN)
- new net: LED97.4 (DOUT), LED99.2 (DIN)
- new net: LED90.2 (DIN), LED92.4 (DOUT)
- new net: LED101.4 (DOUT), LED102.2 (DIN)
- new net: LED100.2 (DIN), LED102.4 (DOUT)
- new net: LED61.4 (DOUT), LED63.2 (DIN)
- new net: LED100.4 (DOUT), LED98.2 (DIN)
- new net: LED96.2 (DIN), LED98.4 (DOUT)
- new net: LED94.2 (DIN), LED96.4 (DOUT)
- new net: LED47.4 (DOUT), LED49.2 (DIN)
- new net: LED85.4 (DOUT), LED87.2 (DIN)
- new net: LED101.2 (DIN), LED99.4 (DOUT)
- new net: LED71.4 (DOUT), LED73.2 (DIN)
- new net: LED92.2 (DIN), LED94.4 (DOUT)
- new net: LED40.2 (DIN), LED42.4 (DOUT)
- new net: LED80.2 (DIN), LED82.4 (DOUT)
